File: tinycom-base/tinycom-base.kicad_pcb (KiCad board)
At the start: 2 copper layers, 45.2 x 45.2 mm, 41 parts, among them J1 MICRO_SD_HINGE, P1 CONN_02X08, P2 CONN_02X08, P3 USB_A, P4 USB_B, U1 SY8008BAAC, U2 SY8008BAAC, U3 SY8008BAAC

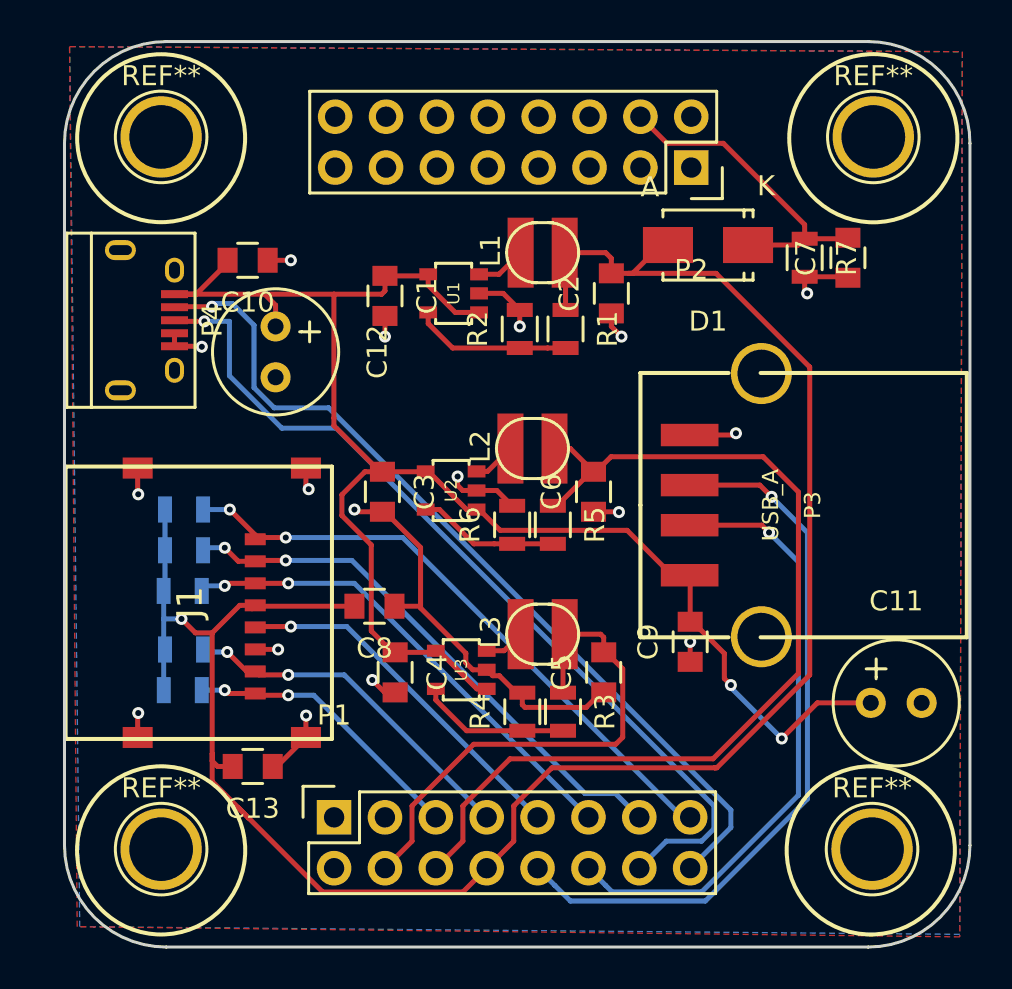
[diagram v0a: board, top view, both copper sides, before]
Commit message: update base board
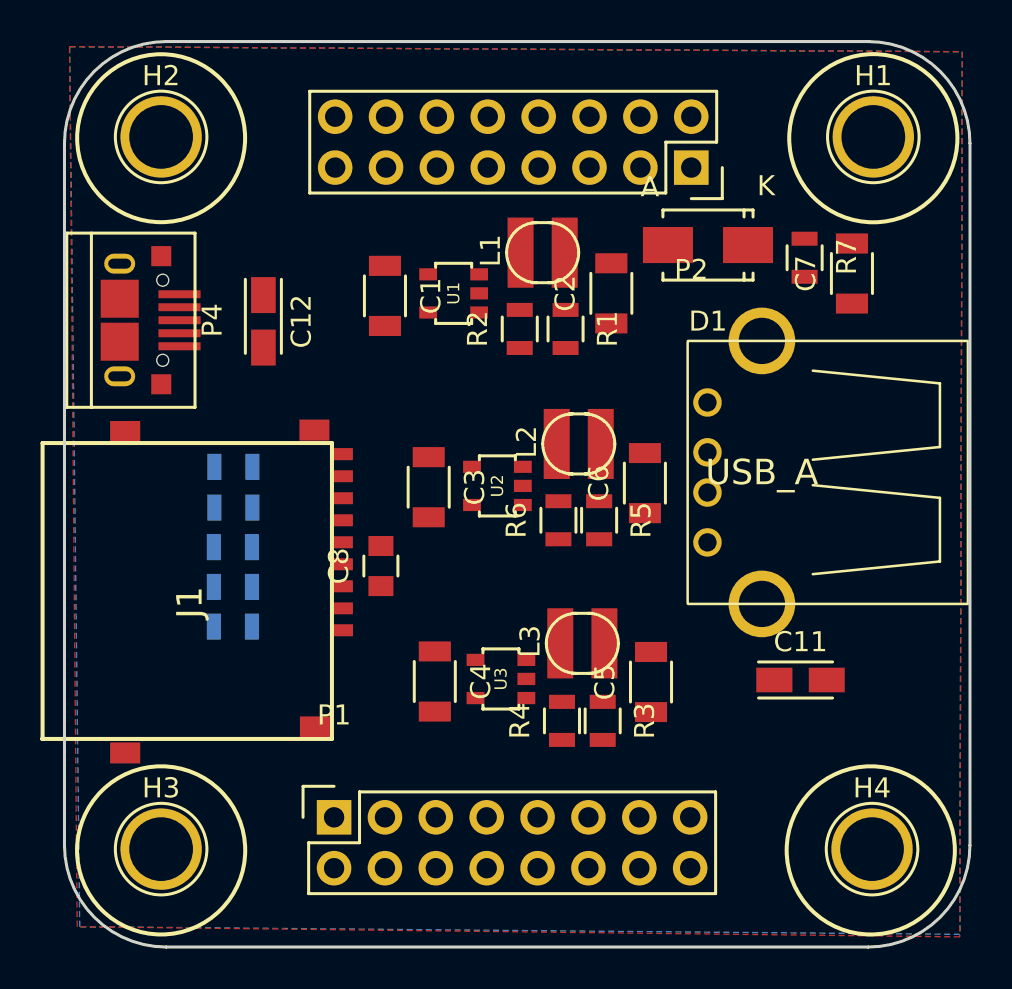
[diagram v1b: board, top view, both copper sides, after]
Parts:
- removed C10, C13, C9: C_Small, Capacitors_SMD:C_0805
- C1, C2, C3, C4, C5, C6, C7: footprint Capacitors_SMD:C_0805 -> Capacitors_SMD:C_1206
- C11, C12: footprint Capacitors_Elko_ThroughHole:Elko_vert_11.2x6.3mm_RM2.5_CopperClear -> Capacitors_Tantalum_SMD:TantalC_SizeA_EIA-3216_Reflow
- J1: footprint armory:MICRO_SD_HINGE_AMP -> tinycom:tc-MICRO_SD_HINGE_AMP
- P3: footprint opendous:USB-A-Receptacle-FCI_87583 -> tinycom:tc-con-usb-USB-A-H
- P4: footprint Connect:USB_Micro-B -> tinycom:tc-USB_Micro-B
- moved R8 4.04 mm to (132.9, 108.5)
- moved R9 3.96 mm to (132.9, 106.5)
- moved C11 3.69 mm to (161.2, 111.1)
- moved R10 3.32 mm to (132.9, 104.5)
- moved R11 3.26 mm to (132.9, 102.5)
- moved R12 3.26 mm to (132.9, 100.5)
- moved P3 2.71 mm to (159.3, 100.8), turned to 180 degrees
- moved C6 2.60 mm to (153.4, 101.3)
- moved C5 2.41 mm to (153.7, 111.2)
- moved C3 2.32 mm to (142.6, 101.5)
- moved L2 2.32 mm to (150.1, 99.3)
- moved R5 2.32 mm to (151.2, 103.1)
- moved R6 2.32 mm to (149.1, 103.1)
- moved U2 2.32 mm to (146.1, 101.4)
- moved C4 2.03 mm to (143.0, 111.2)
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- renumbered REF** to H1, REF** to H2, REF** to H3, REF** to H4
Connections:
- P1 pad 1: UART1_TX -> (no net)
- P1 pad 3: UART1_RX -> (no net)
- P2 pad 1: Net-(P2-Pad1) -> (no net)
- P2 pad 10: Net-(P2-Pad10) -> (no net)
- P2 pad 11: Net-(P2-Pad11) -> (no net)
- P2 pad 12: Net-(P2-Pad12) -> (no net)
- P2 pad 13: Net-(P2-Pad13) -> (no net)
- P2 pad 14: Net-(P2-Pad14) -> (no net)
- P2 pad 15: Net-(P2-Pad15) -> (no net)
- P2 pad 16: Net-(P2-Pad16) -> (no net)
- P2 pad 3: Net-(P2-Pad3) -> (no net)
- P2 pad 5: Net-(P2-Pad5) -> (no net)
- P2 pad 6: Net-(P2-Pad6) -> (no net)
- P2 pad 7: Net-(P2-Pad7) -> (no net)
- P2 pad 8: Net-(P2-Pad8) -> (no net)
- P2 pad 9: Net-(P2-Pad9) -> (no net)
- P4 pad 5: GND -> (no net)
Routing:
- net VCC_33: track 103.0 -> 0.00 mm, vias 1 -> 0
- net +5V: track 82.2 -> 0.00 mm, vias 2 -> 0
- net GND: track 50.2 -> 0.00 mm, vias 17 -> 0
- net VCC_14: track 48.7 -> 0.00 mm
- net UDP0: track 44.3 -> 0.00 mm, vias 1 -> 0
- net UDM0: track 43.9 -> 0.00 mm, vias 1 -> 0
- net UDP1: track 36.4 -> 0.00 mm, vias 1 -> 0
- net SDC0_D2: track 30.9 -> 0.00 mm, vias 2 -> 0
- net UDM1: track 30.8 -> 0.00 mm, vias 1 -> 0
- net SDC0_D3: track 27.4 -> 0.00 mm, vias 2 -> 0
- net VCC_15: track 26.0 -> 0.00 mm
- net SDC0_CMD: track 24.3 -> 0.00 mm, vias 2 -> 0
- net SDC0_CLK: track 18.1 -> 0.00 mm, vias 1 -> 0
- net SDC0_D0: track 17.6 -> 0.00 mm, vias 2 -> 0
- net VCC_30: track 16.3 -> 0.00 mm
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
